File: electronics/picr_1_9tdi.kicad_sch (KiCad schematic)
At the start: 84 parts, among them J1 10118193-0001LF, J2 Conn_01x02_Socket, J3 Conn_01x04_Pin, J4 Conn_01x03_Pin, J5 Conn_01x02_Pin, J6 Conn_01x03_Pin, J7 Conn_01x02_Socket, J8 Conn_01x02_Socket, J9 Conn_01x02_Socket, Q1 BUK6Y10-30PX, U1 DRV8243HQDGQRQ1, U10 215079-4, U11 215079-4, U12 SI8640AB-B-IS1, U13 SI8640AB-B-IS1, U14 MAX12930EASA+, U15 215079-4, U2 CM1223-02SO, U3 TPS62933, U4 DRV8243HQDGQRQ1, U5 MIC5504-3.3YM5, U6 DRV8243HQDGQRQ1, U7 STM32G441KBT6, U8 20021121-00010T4LF, U9 215079-4

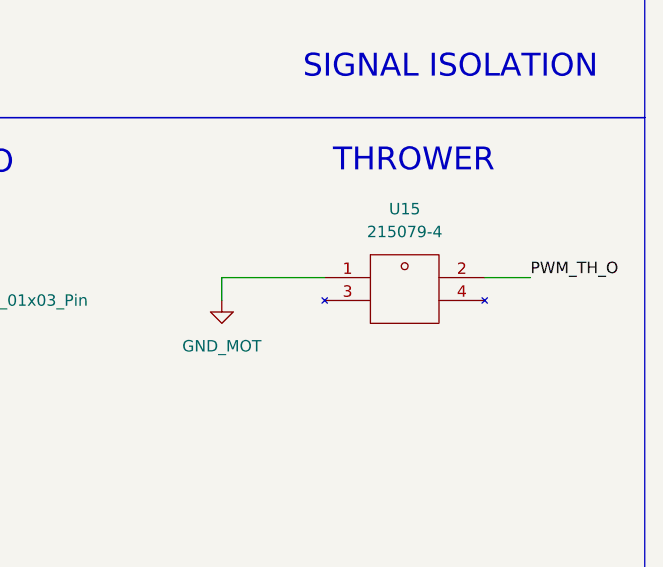
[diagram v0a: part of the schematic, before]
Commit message: .
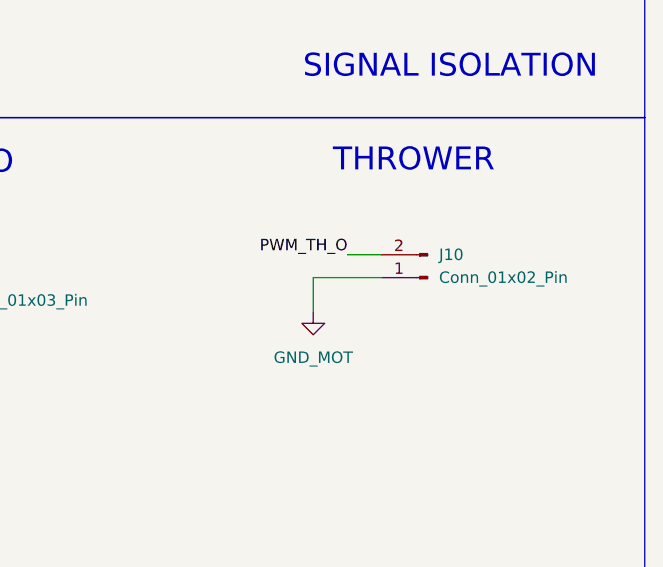
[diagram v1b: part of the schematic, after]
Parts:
- removed U15: 215079-4, Library:TE_Micro-MaTch_215079-4_2x02_P1.27mm_Vertical, symbol Library:215079-4_PWM
- added J10: Conn_01x02_Pin, Connector_PinHeader_2.54mm:PinHeader_1x02_P2.54mm_Vertical, symbol Library:Conn_01x02_Pin
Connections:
- net GND_MOT: now also J10.1 (Pin_1)
- net PWM_TH_O: now also J10.2 (Pin_2)
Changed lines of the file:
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@@
 	(wire
 		(pts
-			(xy 535.94 243.84) (xy 535.94 241.3)
-		)
-		(stroke
-			(width 0)
-			(type default)
-		)
-	)
-	(wire
-		(pts
 			(xy 219.71 280.67) (xy 229.87 280.67)
 		)
@@
 	(wire
 		(pts
-			(xy 425.45 337.82) (xy 441.96 337.82)
+			(xy 546.1 241.3) (xy 553.72 241.3)
 		)
 		(stroke
@@
 	(wire
 		(pts
-			(xy 129.54 143.51) (xy 120.65 143.51)
+			(xy 425.45 337.82) (xy 441.96 337.82)
 		)
 		(stroke
@@
 	(wire
 		(pts
-			(xy 494.03 240.03) (xy 500.38 240.03)
+			(xy 129.54 143.51) (xy 120.65 143.51)
 		)
 		(stroke
@@
 	(wire
 		(pts
-			(xy 26.67 280.67) (xy 36.83 280.67)
+			(xy 494.03 240.03) (xy 500.38 240.03)
 		)
 		(stroke
@@
 	(wire
 		(pts
-			(xy 425.45 278.13) (xy 425.45 292.1)
+			(xy 26.67 280.67) (xy 36.83 280.67)
 		)
 		(stroke
@@
 	(wire
 		(pts
-			(xy 29.21 143.51) (xy 31.75 143.51)
+			(xy 425.45 278.13) (xy 425.45 292.1)
 		)
 		(stroke
@@
 	(wire
 		(pts
-			(xy 66.04 280.67) (xy 66.04 297.18)
+			(xy 29.21 143.51) (xy 31.75 143.51)
 		)
 		(stroke
@@
 	(wire
 		(pts
-			(xy 336.55 297.18) (xy 339.09 297.18)
+			(xy 66.04 280.67) (xy 66.04 297.18)
 		)
 		(stroke
@@
 	(wire
 		(pts
-			(xy 565.15 241.3) (xy 570.23 241.3)
+			(xy 336.55 297.18) (xy 339.09 297.18)
 		)
 		(stroke
@@
 	(wire
 		(pts
-			(xy 535.94 241.3) (xy 547.37 241.3)
-		)
-		(stroke
-			(width 0)
-			(type default)
-		)
-	)
-	(wire
-		(pts
 			(xy 172.72 288.29) (xy 182.88 288.29)
 		)
@@
 	(wire
 		(pts
+			(xy 549.91 238.76) (xy 553.72 238.76)
+		)
+		(stroke
+			(width 0)
+			(type default)
+		)
+	)
+	(wire
+		(pts
 			(xy 127 187.96) (xy 128.27 187.96)
 		)
@@
 	(wire
 		(pts
+			(xy 546.1 245.11) (xy 546.1 241.3)
+		)
+		(stroke
+			(width 0)
+			(type default)
+		)
+	)
+	(wire
+		(pts
 			(xy 185.42 219.71) (xy 190.5 219.71)
 		)
@@
 		)
 	)
+	(label "PWM_TH_O"
+		(at 549.91 238.76 180)
+		(effects
+			(font
+				(size 1.27 1.27)
+			)
+			(justify right bottom)
+		)
+	)
 	(label "PWM_M3_O"
 		(at 474.98 139.7 0)
@@
 		)
 	)
-	(label "PWM_TH_O"
-		(at 570.23 241.3 0)
-		(effects
-			(font
-				(size 1.27 1.27)
-			)
-			(justify left bottom)
-		)
-	)
 	(label "IR_TX"
 		(at 140.97 143.51 0)
@@
 	)
 	(symbol
+		(lib_id "Library:GND")
+		(at 546.1 245.11 0)
+		(unit 1)
+		(exclude_from_sim no)
+		(in_bom yes)
+		(on_board yes)
+		(dnp no)
+		(fields_autoplaced yes)
+		(property "Reference" "#PWR043"
+			(at 546.1 251.46 0)
+			(effects
+				(font
+					(size 1.27 1.27)
+				)
+				(hide yes)
+			)
+		)
+		(property "Value" "GND_MOT"
+			(at 546.1 250.19 0)
+			(effects
+				(font
+					(size 1.27 1.27)
+				)
+			)
+		)
+		(property "Footprint" ""
+			(at 546.1 245.11 0)
+			(effects
+				(font
+					(size 1.27 1.27)
+				)
+				(hide yes)
+			)
+		)
+		(property "Datasheet" ""
+			(at 546.1 245.11 0)
+			(effects
+				(font
+					(size 1.27 1.27)
+				)
+				(hide yes)
+			)
+		)
+		(property "Description" "Power symbol creates a global label with name \"GND\" , ground"
+			(at 546.1 245.11 0)
+			(effects
+				(font
+					(size 1.27 1.27)
+				)
+				(hide yes)
+			)
+		)
+		(pin "1"
+		)
+		(instances
+			(project ""
+				(path "/f4c3b324-9d8f-4d10-8101-dec9d8880fba"
+					(reference "#PWR043")
+					(unit 1)
+				)
+			)
+		)
+	)
+	(symbol
 		(lib_id "Library:+3.3V")
 		(at 511.81 146.05 0)
@@
 	(symbol
 		(lib_id "Library:GND")
-		(at 535.94 243.84 0)
-		(unit 1)
-		(exclude_from_sim no)
-		(in_bom yes)
-		(on_board yes)
-		(dnp no)
-		(fields_autoplaced yes)
-		(property "Reference" "#PWR043"
-			(at 535.94 250.19 0)
-			(effects
-				(font
-					(size 1.27 1.27)
-				)
-				(hide yes)
-			)
-		)
-		(property "Value" "GND_MOT"
-			(at 535.94 248.92 0)
-			(effects
-				(font
-					(size 1.27 1.27)
-				)
-			)
-		)
-		(property "Footprint" ""
-			(at 535.94 243.84 0)
-			(effects
-				(font
-					(size 1.27 1.27)
-				)
-				(hide yes)
-			)
-		)
-		(property "Datasheet" ""
-			(at 535.94 243.84 0)
-			(effects
-				(font
-					(size 1.27 1.27)
-				)
-				(hide yes)
-			)
-		)
-		(property "Description" "Power symbol creates a global label with name \"GND\" , ground"
-			(at 535.94 243.84 0)
-			(effects
-				(font
-					(size 1.27 1.27)
-				)
-				(hide yes)
-			)
-		)
-		(pin "1"
-		)
-		(instances
-			(project "picr_1_9tdi"
-				(path "/f4c3b324-9d8f-4d10-8101-dec9d8880fba"
-					(reference "#PWR043")
-					(unit 1)
-				)
-			)
-		)
-	)
-	(symbol
-		(lib_id "Library:GND")
 		(at 374.65 292.1 0)
 		(unit 1)
@@
 	)
 	(symbol
+		(lib_id "Library:Conn_01x02_Pin")
+		(at 558.8 241.3 180)
+		(unit 1)
+		(exclude_from_sim no)
+		(in_bom yes)
+		(on_board yes)
+		(dnp no)
+		(fields_autoplaced yes)
+		(property "Reference" "J10"
+			(at 560.07 238.7599 0)
+			(effects
+				(font
+					(size 1.27 1.27)
+				)
+				(justify right)
+			)
+		)
+		(property "Value" "Conn_01x02_Pin"
+			(at 560.07 241.2999 0)
+			(effects
+				(font
+					(size 1.27 1.27)
+				)
+				(justify right)
+			)
+		)
+		(property "Footprint" "Connector_PinHeader_2.54mm:PinHeader_1x02_P2.54mm_Vertical"
+			(at 558.8 241.3 0)
+			(effects
+				(font
+					(size 1.27 1.27)
+				)
+				(hide yes)
+			)
+		)
+		(property "Datasheet" "~"
+			(at 558.8 241.3 0)
+			(effects
+				(font
+					(size 1.27 1.27)
+				)
+				(hide yes)
+			)
+		)
+		(property "Description" "Generic connector, single row, 01x02, script generated"
+			(at 558.8 241.3 0)
+			(effects
+				(font
+					(size 1.27 1.27)
+				)
+				(hide yes)
+			)
+		)
+		(pin "2"
+		)
+		(pin "1"
+		)
+		(instances
+			(project "picr_1_9tdi"
+				(path "/f4c3b324-9d8f-4d10-8101-dec9d8880fba"
+					(reference "J10")
+					(unit 1)
+				)
+			)
+		)
+	)
+	(symbol
 		(lib_id "Library:215079-4_2")
 		(at 450.85 294.64 0)
@@
 					(unit 1)
 				)
-			)
-		)
-	)
-	(symbol
-		(lib_id "Library:215079-4_PWM")
-		(at 557.53 243.84 0)
-		(unit 1)
-		(exclude_from_sim no)
-		(in_bom yes)
-		(on_board yes)
-		(dnp no)
-		(fields_autoplaced yes)
-		(property "Reference" "U15"
-			(at 556.26 233.68 0)
-			(effects
-				(font
-					(size 1.27 1.27)
-				)
-			)
-		)
-		(property "Value" "215079-4"
-			(at 556.26 236.22 0)
-			(effects
-				(font
-					(size 1.27 1.27)
-				)
-			)
-		)
-		(property "Footprint" "Library:TE_Micro-MaTch_215079-4_2x02_P1.27mm_Vertical"
-			(at 553.466 255.016 0)
-			(effects
-				(font
-					(size 1.27 1.27)
-				)
-				(hide yes)
-			)
-		)
-		(property "Datasheet" "https://atta.szlcsc.com/upload/public/pdf/source/20181106/C306160_C0F6687678D8320B9FEA0BB065D7ACFE.pdf"
-			(at 551.942 253.746 0)
-			(do_not_autoplace yes)
-			(effects
-				(font
-					(size 1.27 1.27)
-				)
-				(hide yes)
-			)
-		)
-		(property "Description" "Pins Structure:2x2P Pitch:2.54mm Mounting Style:Direct Insert Reference Series:- Number of Pins:4P Number of Rows:2 Number of PINs Per Row:2 Row Spacing:2.54mm Contact Material:Phosphor Bronze Contact Plating:Tin Operating Temperature Range:-40°C~+105°C Ope"
-			(at 556.514 255.778 0)
-			(effects
-				(font
-					(size 1.27 1.27)
-				)
-				(hide yes)
-			)
-		)
-		(property "Manufacturer Part" "215079-4"
-			(at 557.784 247.904 0)
-			(effects
-				(font
-					(size 1 1)
-				)
-				(hide yes)
-			)
-		)
-		(property "Manufacturer" "TE Connectivity(泰科电子)"
-			(at 556.514 259.334 0)
-			(effects
-				(font
-					(size 1.27 1.27)
-				)
-				(hide yes)
-			)
-		)
-		(property "Supplier Part" "C306232"
-			(at 554.736 254.254 0)
-			(effects
-				(font
-					(size 1.27 1.27)
-				)
-				(hide yes)
-			)
-		)
-		(property "Supplier" "LCSC"
-			(at 549.148 254.254 0)
-			(effects
-				(font
-					(size 1.27 1.27)
-				)
-				(hide yes)
-			)
-		)
-		(property "LCSC Part Name" "215079-4"
-			(at 555.752 253.238 0)
-			(effects
-				(font
-					(size 1.27 1.27)
-				)
-				(hide yes)
-			)
-		)
-		(pin "1"
-		)
-		(pin "3"
-		)
-		(pin "4"
-		)
-		(pin "2"
-		)
-		(instances
-			(project ""
-				(path "/f4c3b324-9d8f-4d10-8101-dec9d8880fba"
-					(reference "U15")
-					(unit 1)
-				)

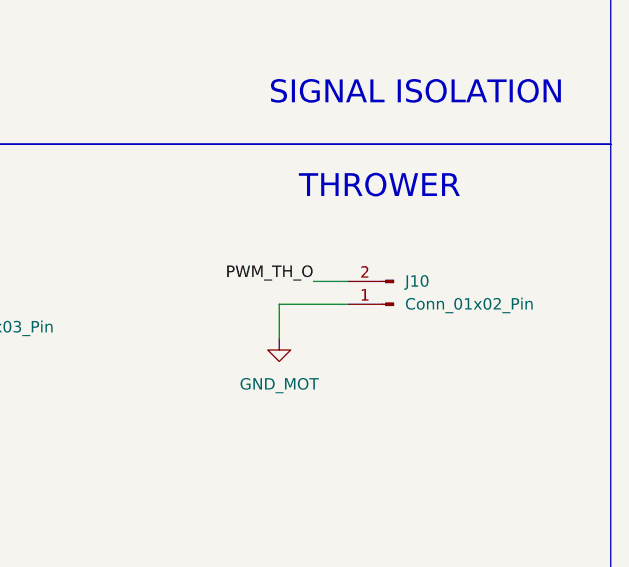
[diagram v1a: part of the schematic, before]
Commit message: .
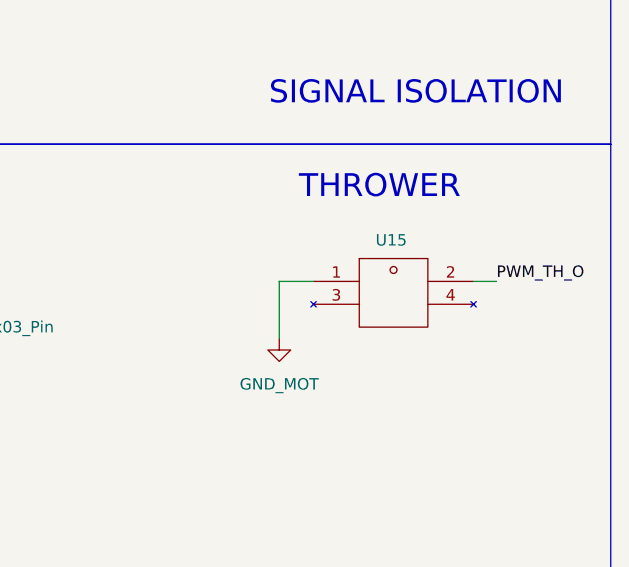
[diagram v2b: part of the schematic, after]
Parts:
- removed J10: Conn_01x02_Pin, Connector_PinHeader_2.54mm:PinHeader_1x02_P2.54mm_Vertical, symbol Library:Conn_01x02_Pin
- added U15: ~, Library:TE_Micro-MaTch_215079-4_2x02_P1.27mm_Vertical, symbol Library:215079-4_PWM
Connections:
- net GND_MOT: now also U15.1
- net PWM_TH_O: now also U15.2
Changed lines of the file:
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@@
 	(wire
 		(pts
+			(xy 546.1 238.76) (xy 549.91 238.76)
+		)
+		(stroke
+			(width 0)
+			(type default)
+		)
+	)
+	(wire
+		(pts
 			(xy 233.68 341.63) (xy 236.22 341.63)
 		)
@@
 	(wire
 		(pts
+			(xy 570.23 238.76) (xy 567.69 238.76)
+		)
+		(stroke
+			(width 0)
+			(type default)
+		)
+	)
+	(wire
+		(pts
 			(xy 472.44 144.78) (xy 488.95 144.78)
 		)
@@
 	(wire
 		(pts
-			(xy 546.1 241.3) (xy 553.72 241.3)
-		)
-		(stroke
-			(width 0)
-			(type default)
-		)
-	)
-	(wire
-		(pts
 			(xy 425.45 337.82) (xy 441.96 337.82)
 		)
@@
 	(wire
 		(pts
-			(xy 549.91 238.76) (xy 553.72 238.76)
-		)
-		(stroke
-			(width 0)
-			(type default)
-		)
-	)
-	(wire
-		(pts
 			(xy 127 187.96) (xy 128.27 187.96)
 		)
@@
 	(wire
 		(pts
-			(xy 546.1 245.11) (xy 546.1 241.3)
+			(xy 546.1 238.76) (xy 546.1 245.11)
 		)
 		(stroke
@@
 		)
 	)
-	(label "PWM_TH_O"
-		(at 549.91 238.76 180)
-		(effects
-			(font
-				(size 1.27 1.27)
-			)
-			(justify right bottom)
-		)
-	)
 	(label "PWM_M3_O"
 		(at 474.98 139.7 0)
@@
 		)
 	)
+	(label "PWM_TH_O"
+		(at 570.23 238.76 0)
+		(effects
+			(font
+				(size 1.27 1.27)
+			)
+			(justify left bottom)
+		)
+	)
 	(label "PWM_TH_I"
 		(at 444.5 142.24 180)
@@
 	)
 	(symbol
+		(lib_id "Library:215079-4_PWM")
+		(at 560.07 241.3 0)
+		(unit 1)
+		(exclude_from_sim no)
+		(in_bom yes)
+		(on_board yes)
+		(dnp no)
+		(property "Reference" "U15"
+			(at 558.546 234.188 0)
+			(effects
+				(font
+					(size 1.27 1.27)
+				)
+			)
+		)
+		(property "Value" "~"
+			(at 558.8 233.68 0)
+			(effects
+				(font
+					(size 1.27 1.27)
+				)
+				(hide yes)
+			)
+		)
+		(property "Footprint" "Library:TE_Micro-MaTch_215079-4_2x02_P1.27mm_Vertical"
+			(at 556.006 252.476 0)
+			(effects
+				(font
+					(size 1.27 1.27)
+				)
+				(hide yes)
+			)
+		)
+		(property "Datasheet" "https://atta.szlcsc.com/upload/public/pdf/source/20181106/C306160_C0F6687678D8320B9FEA0BB065D7ACFE.pdf"
+			(at 554.482 251.206 0)
+			(do_not_autoplace yes)
+			(effects
+				(font
+					(size 1.27 1.27)
+				)
+				(hide yes)
+			)
+		)
+		(property "Description" "Pins Structure:2x2P Pitch:2.54mm Mounting Style:Direct Insert Reference Series:- Number of Pins:4P Number of Rows:2 Number of PINs Per Row:2 Row Spacing:2.54mm Contact Material:Phosphor Bronze Contact Plating:Tin Operating Temperature Range:-40°C~+105°C Ope"
+			(at 559.054 253.238 0)
+			(effects
+				(font
+					(size 1.27 1.27)
+				)
+				(hide yes)
+			)
+		)
+		(property "Manufacturer Part" "215079-4"
+			(at 560.324 245.364 0)
+			(effects
+				(font
+					(size 1 1)
+				)
+				(hide yes)
+			)
+		)
+		(property "Manufacturer" "TE Connectivity(泰科电子)"
+			(at 559.054 256.794 0)
+			(effects
+				(font
+					(size 1.27 1.27)
+				)
+				(hide yes)
+			)
+		)
+		(property "Supplier Part" "C306232"
+			(at 557.276 251.714 0)
+			(effects
+				(font
+					(size 1.27 1.27)
+				)
+				(hide yes)
+			)
+		)
+		(property "Supplier" "LCSC"
+			(at 551.688 251.714 0)
+			(effects
+				(font
+					(size 1.27 1.27)
+				)
+				(hide yes)
+			)
+		)
+		(property "LCSC Part Name" "215079-4"
+			(at 558.292 250.698 0)
+			(effects
+				(font
+					(size 1.27 1.27)
+				)
+				(hide yes)
+			)
+		)
+		(pin "2"
+		)
+		(pin "1"
+		)
+		(pin "3"
+		)
+		(pin "4"
+		)
+		(instances
+			(project ""
+				(path "/f4c3b324-9d8f-4d10-8101-dec9d8880fba"
+					(reference "U15")
+					(unit 1)
+				)
+			)
+		)
+	)
+	(symbol
 		(lib_id "Library:GND")
 		(at 219.71 360.68 0)
@@
 					(unit 1)
 				)
-			)
-		)
-	)
-	(symbol
-		(lib_id "Library:Conn_01x02_Pin")
-		(at 558.8 241.3 180)
-		(unit 1)
-		(exclude_from_sim no)
-		(in_bom yes)
-		(on_board yes)
-		(dnp no)
-		(fields_autoplaced yes)
-		(property "Reference" "J10"
-			(at 560.07 238.7599 0)
-			(effects
-				(font
-					(size 1.27 1.27)
-				)
-				(justify right)
-			)
-		)
-		(property "Value" "Conn_01x02_Pin"
-			(at 560.07 241.2999 0)
-			(effects
-				(font
-					(size 1.27 1.27)
-				)
-				(justify right)
-			)
-		)
-		(property "Footprint" "Connector_PinHeader_2.54mm:PinHeader_1x02_P2.54mm_Vertical"
-			(at 558.8 241.3 0)
-			(effects
-				(font
-					(size 1.27 1.27)
-				)
-				(hide yes)
-			)
-		)
-		(property "Datasheet" "~"
-			(at 558.8 241.3 0)
-			(effects
-				(font
-					(size 1.27 1.27)
-				)
-				(hide yes)
-			)
-		)
-		(property "Description" "Generic connector, single row, 01x02, script generated"
-			(at 558.8 241.3 0)
-			(effects
-				(font
-					(size 1.27 1.27)
-				)
-				(hide yes)
-			)
-		)
-		(pin "2"
-		)
-		(pin "1"
-		)
-		(instances
-			(project "picr_1_9tdi"
-				(path "/f4c3b324-9d8f-4d10-8101-dec9d8880fba"
-					(reference "J10")
-					(unit 1)
-				)

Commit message: .
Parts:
- J3: footprint Connector_PinHeader_2.54mm:PinHeader_1x04_P2.54mm_Vertical -> Library:PinHeader_1x04_P2.54mm_Vertical
- J4, J6: footprint Connector_PinHeader_2.54mm:PinHeader_1x03_P2.54mm_Vertical -> Library:PinHeader_1x03_P2.54mm_Vertical
- J5: footprint Connector_PinHeader_2.54mm:PinHeader_1x02_P2.54mm_Vertical -> Library:PinHeader_1x02_P2.54mm_Vertical
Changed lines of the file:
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@@
 			)
 		)
-		(property "Footprint" "Connector_PinHeader_2.54mm:PinHeader_1x03_P2.54mm_Vertical"
+		(property "Footprint" "Library:PinHeader_1x03_P2.54mm_Vertical"
 			(at 505.46 242.57 0)
 			(effects
@@
 			)
 		)
-		(property "Footprint" "Connector_PinHeader_2.54mm:PinHeader_1x03_P2.54mm_Vertical"
+		(property "Footprint" "Library:PinHeader_1x03_P2.54mm_Vertical"
 			(at 450.85 241.3 0)
 			(effects
@@
 			)
 		)
-		(property "Footprint" "Connector_PinHeader_2.54mm:PinHeader_1x04_P2.54mm_Vertical"
+		(property "Footprint" "Library:PinHeader_1x04_P2.54mm_Vertical"
 			(at 447.04 342.9 0)
 			(effects
@@
 			)
 		)
-		(property "Footprint" "Connector_PinHeader_2.54mm:PinHeader_1x02_P2.54mm_Vertical"
+		(property "Footprint" "Library:PinHeader_1x02_P2.54mm_Vertical"
 			(at 481.33 341.63 0)
 			(effects
